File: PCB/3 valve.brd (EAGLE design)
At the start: 127 x 44.4 mm, 27 parts, among them T1 2N2222, T2 2N2222, T3 2N2222, T4 2N2222, T5 2N2222

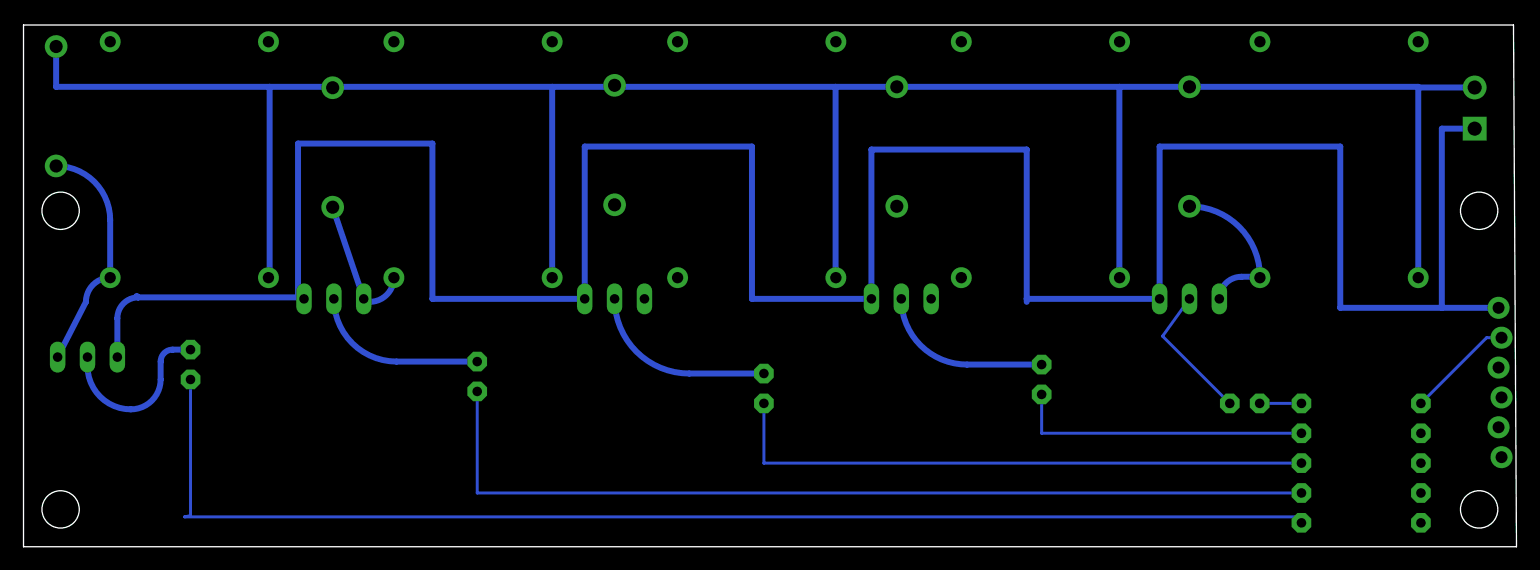
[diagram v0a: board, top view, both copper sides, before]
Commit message: board updates
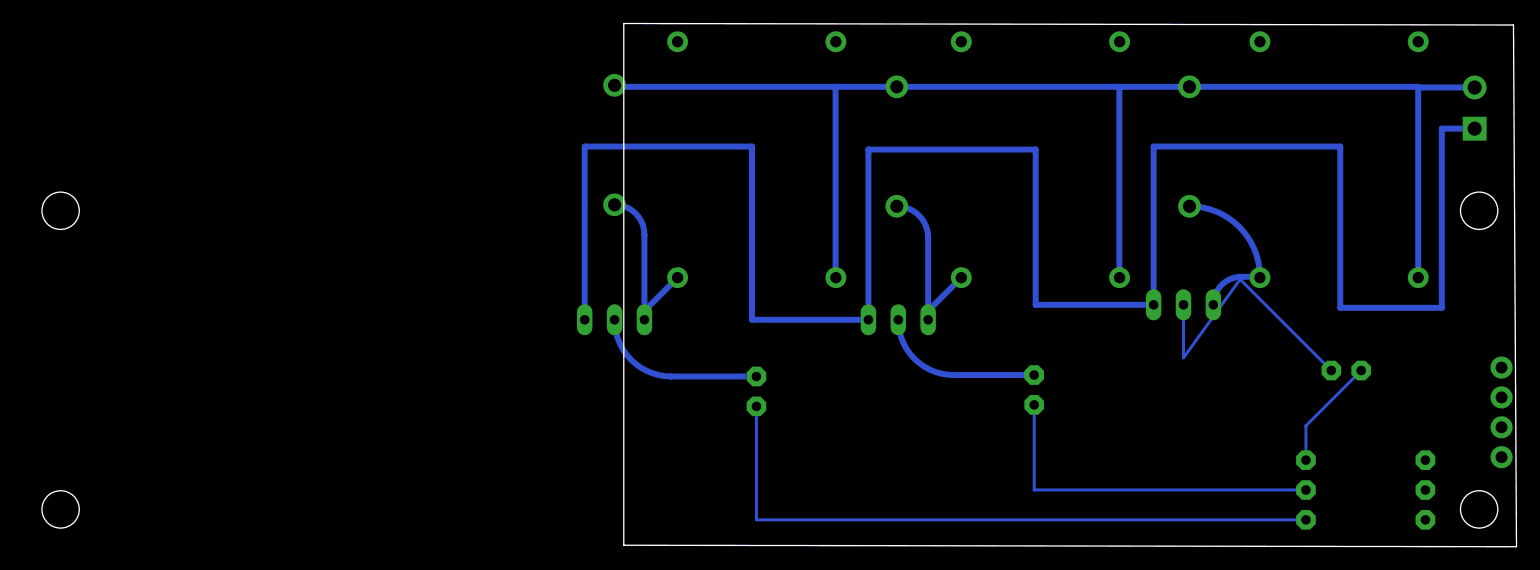
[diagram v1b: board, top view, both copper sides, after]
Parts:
- removed D4, D5: 1N4004, adafruit:DO41-10
- removed LED4, LED5: (no value), adafruit:LED5MM
- removed R4, R5: (no value), adafruit:0207/10
- removed T4, T5: 2N2222, adafruit:TO92-EBC-OVAL
- removed U$5: (no value), local eagle library:VALVTEST2
- removed VALVE4: 4, local eagle library:VALVTEST2
- SV1: device SparkFun-Connectors:1X06_LOCK -> SparkFun-Connectors:1X04
- moved LED1 9.08 mm to (211.1, 15.0)
- moved R1 4.84 mm to (212.7, 7.37)
- moved R3 4.84 mm to (212.7, 2.29)
- moved R2 4.84 mm to (212.7, 4.83)
- moved T2 1.80 mm to (173.0, 18.0)
- moved T3 1.78 mm to (148.8, 18.0)
- moved LED2 1.09 mm to (184.5, 13.3)
- moved T1 0.72 mm to (197.2, 19.3)
- moved LED3 0.68 mm to (160.9, 13.2)
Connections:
- removed net N$12: LED4.A, R4.2
- removed net N$13: D5.A, T5.C, U$5.PAD11
- removed net N$14: LED5.K, T5.B
- removed net N$15: LED5.A, R5.2
- removed net N$4: D4.A, T4.C, VALVE4.PAD11
- removed net N$43: R4.1, SV1.2
- removed net N$45: R5.1, SV1.1
- removed net N$8: LED4.K, T4.B
- net 5V: no longer D4.C, D5.C, U$5.PAD10, VALVE4.PAD10
- net GND: now also SV1.4; no longer SV1.6, T4.E, T5.E
- net N$19: now also SV1.1; no longer SV1.3
- net N$30: now also SV1.3; no longer SV1.5
- net N$44: now also SV1.2; no longer SV1.4
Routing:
- net N$15: track 107.3 -> 0.00 mm
- net 5V: track 205.6 -> 122.3 mm
- net N$12: track 78.7 -> 0.00 mm
- net GND: track 244.4 -> 175.3 mm
- net N$13: track 19.6 -> 0.00 mm
- net N$9: track 0.00 -> 15.6 mm
- net N$5: track 0.00 -> 15.5 mm
- net N$8: track 14.4 -> 0.00 mm
- net N$14: track 14.0 -> 0.00 mm
- net N$2: track 12.0 -> 23.7 mm
- net N$4: track 11.1 -> 0.00 mm
- net N$30: track 9.17 -> 0.00 mm
- net N$3: track 3.56 -> 9.57 mm
- net N$11: track 50.8 -> 56.4 mm
- net N$7: track 25.4 -> 30.4 mm
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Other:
- board size 127 x 44.4 mm -> 75.9 x 44.5 mm
